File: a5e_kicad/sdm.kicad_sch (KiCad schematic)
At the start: 22 parts, among them U2 W25X20CLZP, U7 A5EB013B-B23B

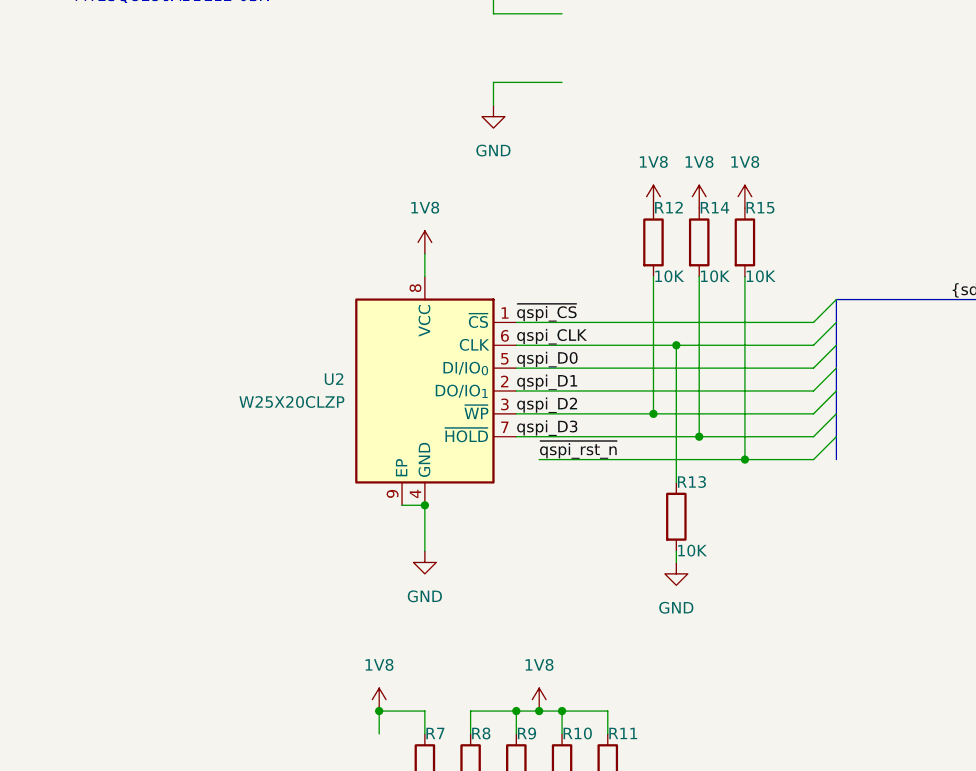
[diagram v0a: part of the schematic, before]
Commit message: savegame
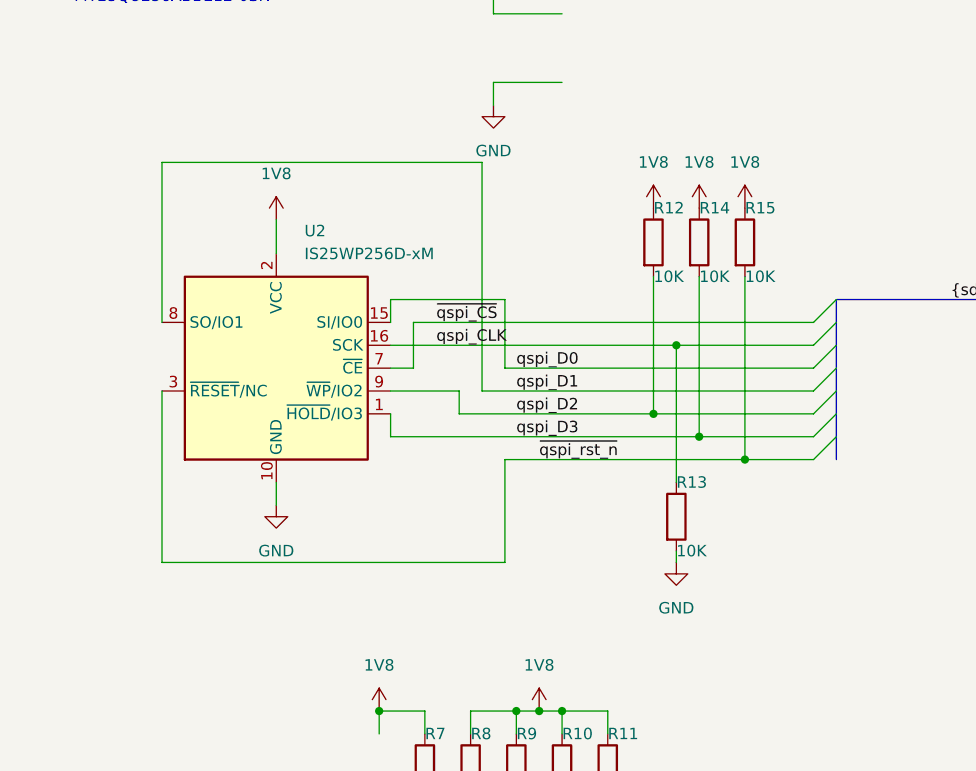
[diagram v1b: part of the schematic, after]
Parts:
- removed U2: W25X20CLZP, Package_SON:WSON-8-1EP_6x5mm_P1.27mm_EP3.4x4.3mm, symbol Memory_Flash:W25X20CLZP
- added U2: IS25WP256D-xM, Package_SO:SOIC-16W_7.5x10.3mm_P1.27mm, symbol Memory_Flash:IS25WP256D-xM
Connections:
- net 1V8: now also U2.2 (VCC)
- net GND: now also U2.10 (GND)
- net qspi_CLK: now also U2.16 (SCK)
- net qspi_D0: now also U2.15 (SI/IO0)
- net qspi_D1: now also U2.8 (SO/IO1)
- net qspi_D2: now also U2.9 (~{WP}/IO2)
- net qspi_D3: now also U2.1 (~{HOLD}/IO3)
- net ~{qspi_CS}: now also U2.7 (~{CE})
- net ~{qspi_rst_n}: now also U2.3 (~{RESET}/NC)
